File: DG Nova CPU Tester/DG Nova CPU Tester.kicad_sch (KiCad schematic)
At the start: 122 parts, among them J1 Slot_02x50_Odd_Even, J10 Programmed I/O, J11 CPU Option Inputs, J12 Data Channel, J13 Program Interrupt, J14 System Control, J17 CPU Option Outputs, J18 MEM Control Outputs, J19 Logic 8 CH, J20 Logic 8 CH, J21 Arduino Anolog Pins, J22 Arduino Digital Pins, J23 Arduino Digital Pins, J4 ATX Power Port, J6 MBO, J7 MEM, J8 Data Channel, J9 Front Panel Controls, SW1 Arduino Mega Reset, SW1 Pico Reset, SW2 Power Swtich, U1 74HC14, U2 Pico

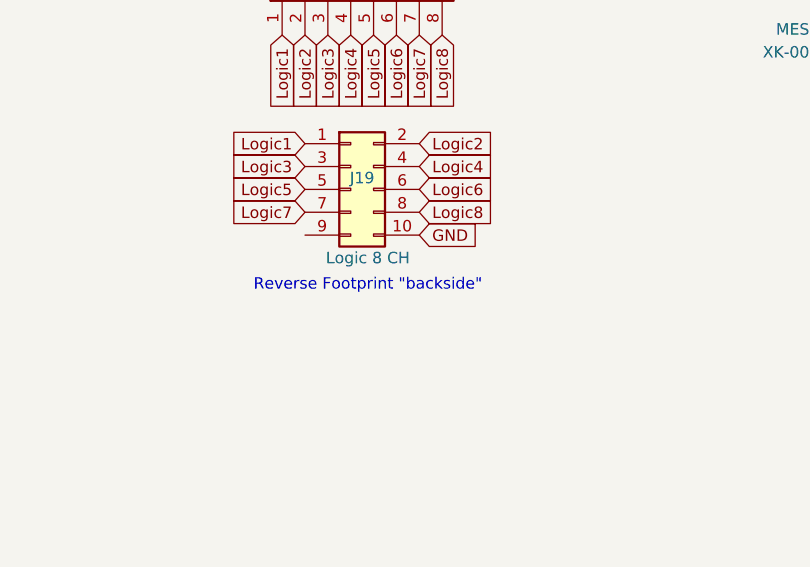
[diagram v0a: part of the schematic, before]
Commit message: Updates
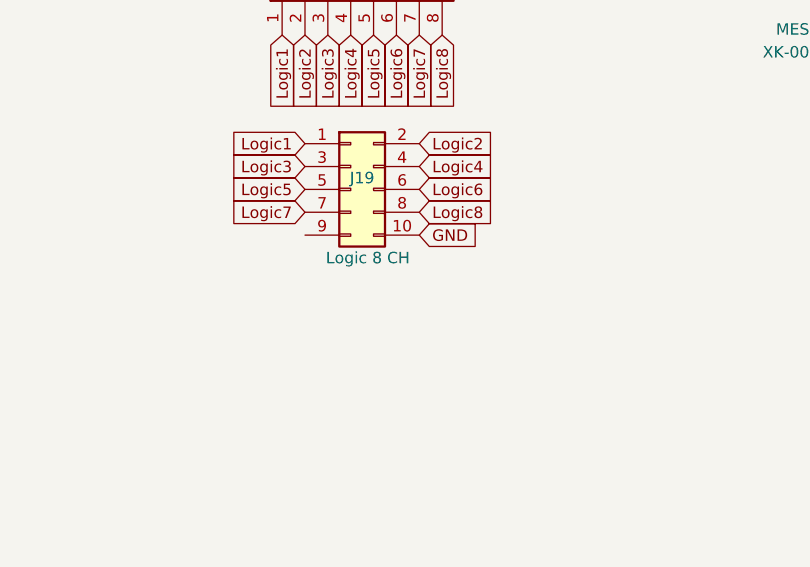
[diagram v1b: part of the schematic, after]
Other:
- note removed: "Reverse Footprint "backside""
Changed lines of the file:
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@@
-    (effects (font (size 1.27 1.27)) (justify left bottom))
-  )
-  (text "Reverse Footprint \"backside\"" (at 278.765 111.76 0)
     (effects (font (size 1.27 1.27)) (justify left bottom))
   )

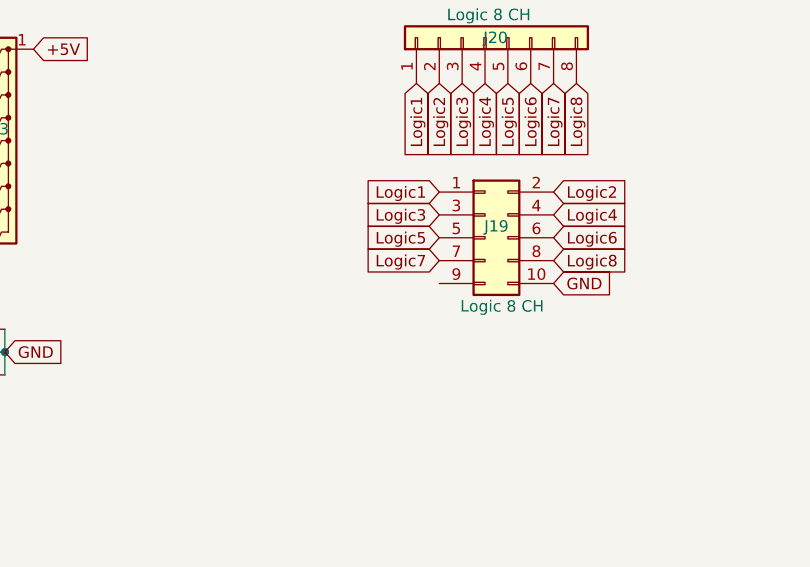
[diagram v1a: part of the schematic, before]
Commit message: QuantX schematic update
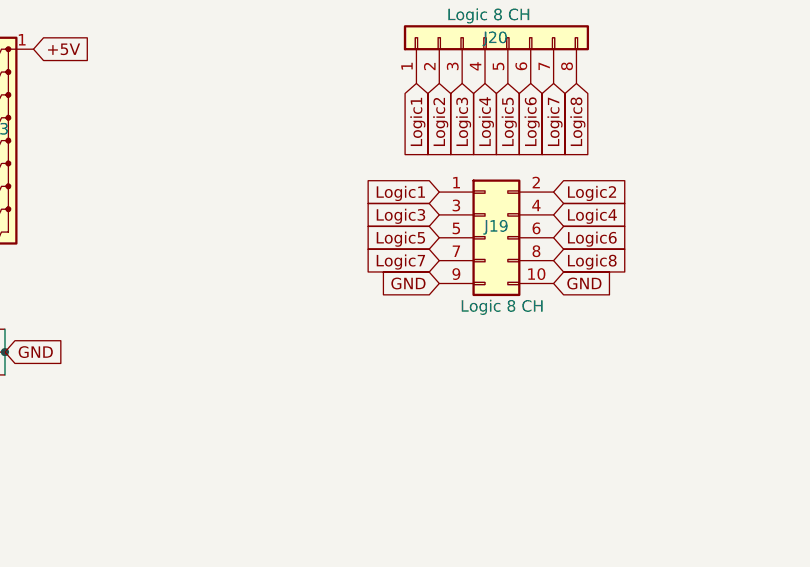
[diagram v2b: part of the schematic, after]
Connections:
- net GND: now also J19.9 (Pin_9)
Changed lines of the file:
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@@
+    )
+  )
+  (global_label "GND" (shape input) (at 284.48 105.41 180) (fields_autoplaced)
+    (effects (font (size 1.27 1.27)) (justify right))
+    (property "Intersheetrefs" "${INTERSHEET_REFS}" (at 278.2785 105.41 0)
+      (effects (font (size 1.27 1.27)) (justify right) hide)
     )
   )
